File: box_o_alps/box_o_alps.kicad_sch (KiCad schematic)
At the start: 69 parts, among them SW00 SW_Push, SW01 SW_Push, SW02 SW_Push, SW03 SW_Push, SW04 SW_Push, SW05 SW_Push, SW06 SW_Push, SW07 SW_Push, SW08 SW_Push, SW09 SW_Push, SW10 SW_Push, SW11 SW_Push, SW12 SW_Push, SW13 SW_Push, SW14 SW_Push, SW15 SW_Push, SW16 SW_Push, SW17 SW_Push, SW18 SW_Push, SW19 SW_Push, SW20 SW_Push, SW21 SW_Push, SW22 SW_Push, SW23 SW_Push, SW24 SW_Push, SW25 SW_Push, SW26 SW_Push, SW27 SW_Push, SW28 SW_Push, SW29 SW_Push, SW33 SW_Push, SW34 SW_Push, SW35 SW_Push, SW36 SW_Push, U00 BlackPill_STLINK

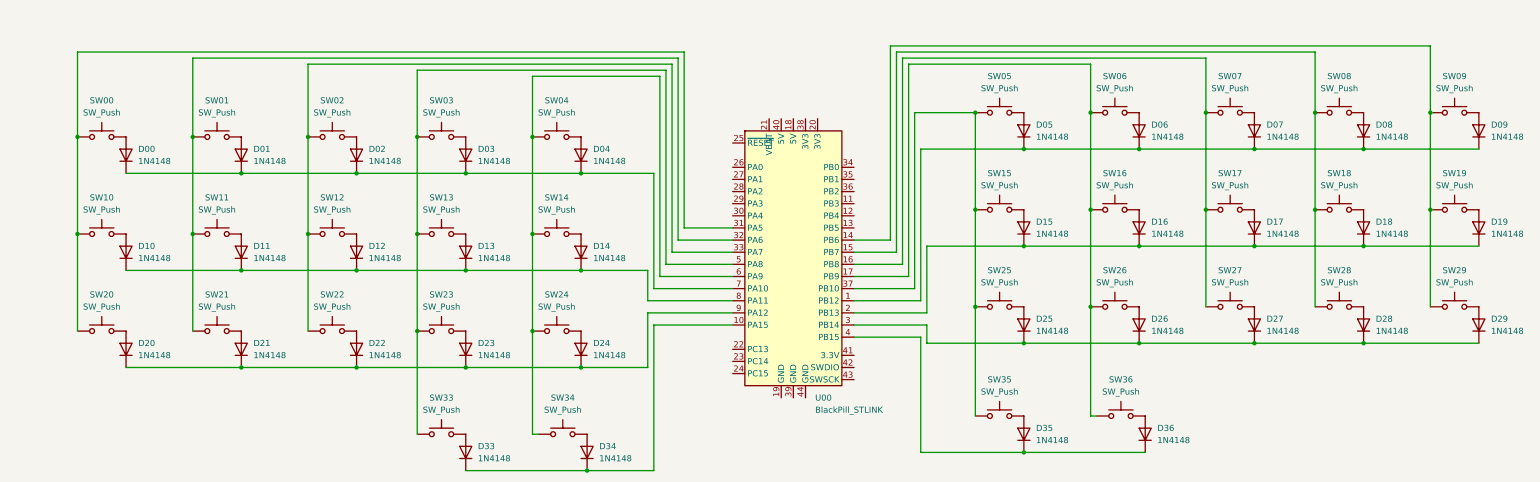
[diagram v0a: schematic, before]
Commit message: Too lazy to comment
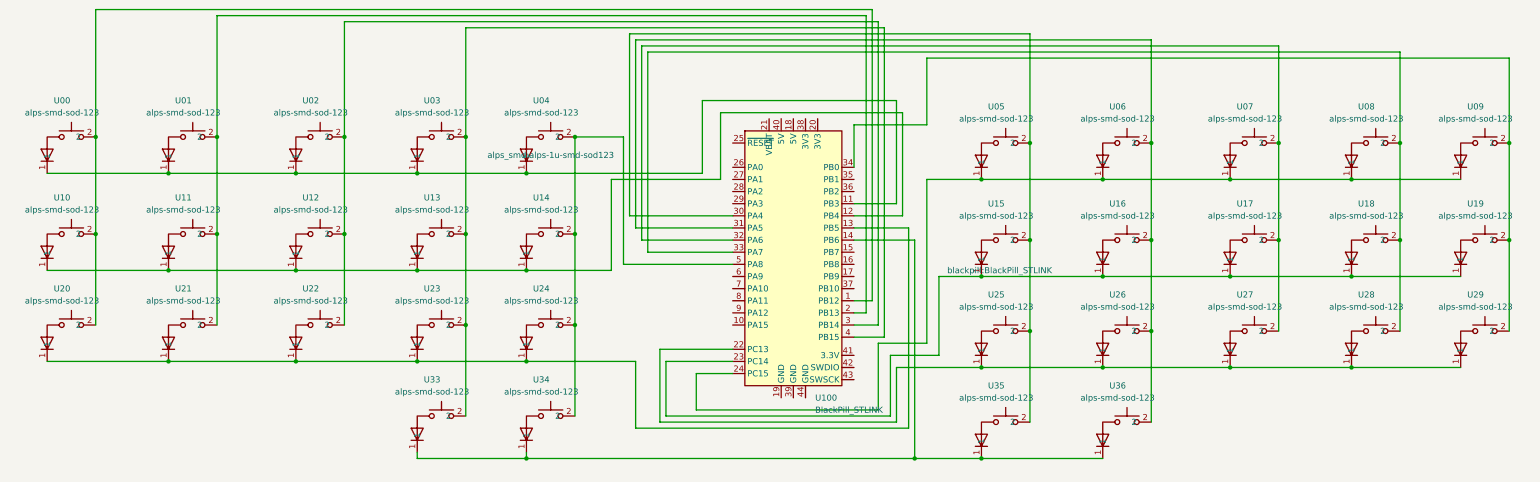
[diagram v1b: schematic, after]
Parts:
- removed D00, D01, D02, D03, D04, D05, D06, D07, D08, D09, D10, D11, D12, D13, D14, D15, D16, D17, D18, D19, D20, D21, D22, D23, D24, D25, D26, D27, D28, D29, D33, D34, D35, D36: 1N4148, Diode_SMD:D_SOD-123, symbol Diode:1N4148
- removed SW00, SW01, SW02, SW03, SW04, SW05, SW06, SW07, SW08, SW09, SW10, SW11, SW12, SW13, SW14, SW15, SW16, SW17, SW18, SW19, SW20, SW21, SW22, SW23, SW24, SW25, SW26, SW27, SW28, SW29: SW_Push, Button_Switch_Keyboard:SW_Matias_1.00u, symbol Switch:SW_Push
- removed SW33, SW34, SW35, SW36: SW_Push, Button_Switch_Keyboard:SW_Matias_1.50u, symbol Switch:SW_Push
- added U00, U01, U02, U03, U04, U05, U06, U07, U08, U09, U10, U11, U12, U13, U14, U15, U16, U17, U18, U19, U20, U21, U22, U23, U24, U25, U26, U27, U28, U29, U33, U34, U35, U36: alps-smd-sod-123, alps_smd:alps-1u-smd-sod123, symbol alps-smd:alps-smd-sod-123
- renumbered U00 to U100
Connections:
- net at U100.1 (PB12): now also U00.2, U10.2, U20.2
- net at U100.3 (PB14): now also U02.2, U12.2, U22.2
- net at U100.33 (PA7): now also U08.2, U18.2, U28.2
- net at U100.4 (PB15): now also U03.2, U13.2, U23.2, U33.2
- net at U100.14 (PB6): now also U33.1, U34.1, U35.1, U36.1
- net at U100.5 (PA8): now also U04.2, U14.2, U24.2, U34.2
- net at U100.2 (PB13): now also U01.2, U11.2, U21.2
- net at U100.32 (PA6): now also U07.2, U17.2, U27.2
- net at U100.31 (PA5): now also U06.2, U16.2, U26.2, U36.2
- net at U100.11 (PB3): now also U00.1, U01.1, U02.1, U03.1, U04.1
- net at U100.12 (PB4): now also U10.1, U11.1, U12.1, U13.1, U14.1
- net at U100.13 (PB5): now also U20.1, U21.1, U22.1, U23.1, U24.1
- net at U100.22 (PC13): now also U25.1, U26.1, U27.1, U28.1, U29.1
- net at U100.23 (PC14): now also U15.1, U16.1, U17.1, U18.1, U19.1
- net at U100.24 (PC15): now also U05.1, U06.1, U07.1, U08.1, U09.1
- net at U100.30 (PA4): now also U05.2, U15.2, U25.2, U35.2
- net at U100.34 (PB0): now also U09.2, U19.2, U29.2
